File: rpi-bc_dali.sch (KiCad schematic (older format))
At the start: 5 parts, among them J1 Raspberry_Pi_2_3, J2 Conn_01x04, J3 Conn_01x04, J4 Conn_01x04, J5 Conn_01x04

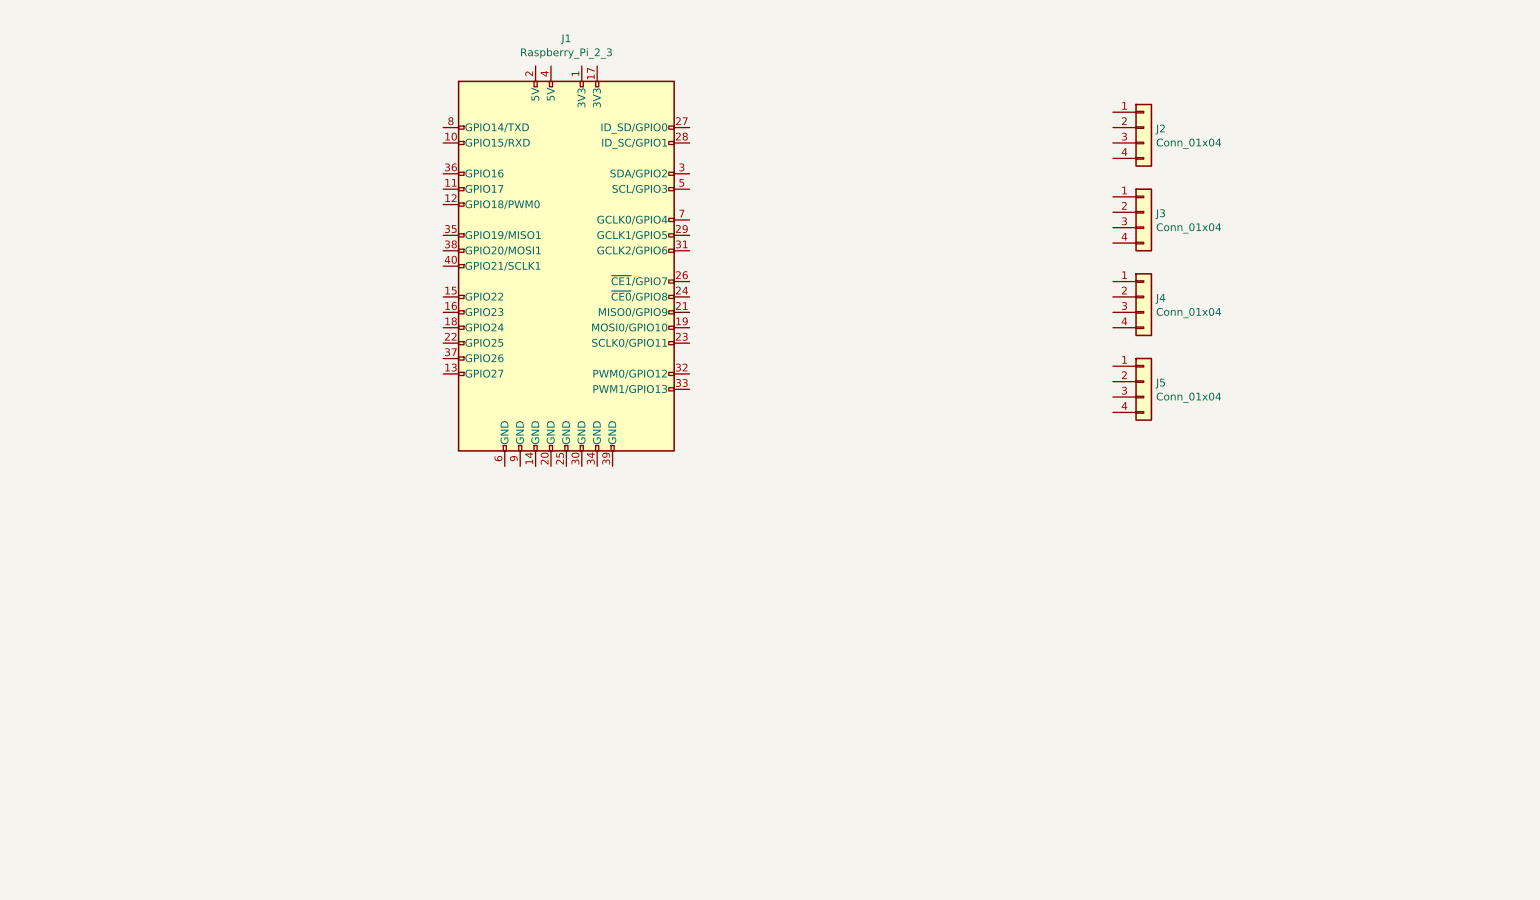
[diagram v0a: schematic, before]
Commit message: master : schematic update
 - first pass schematic.
 - annotated.
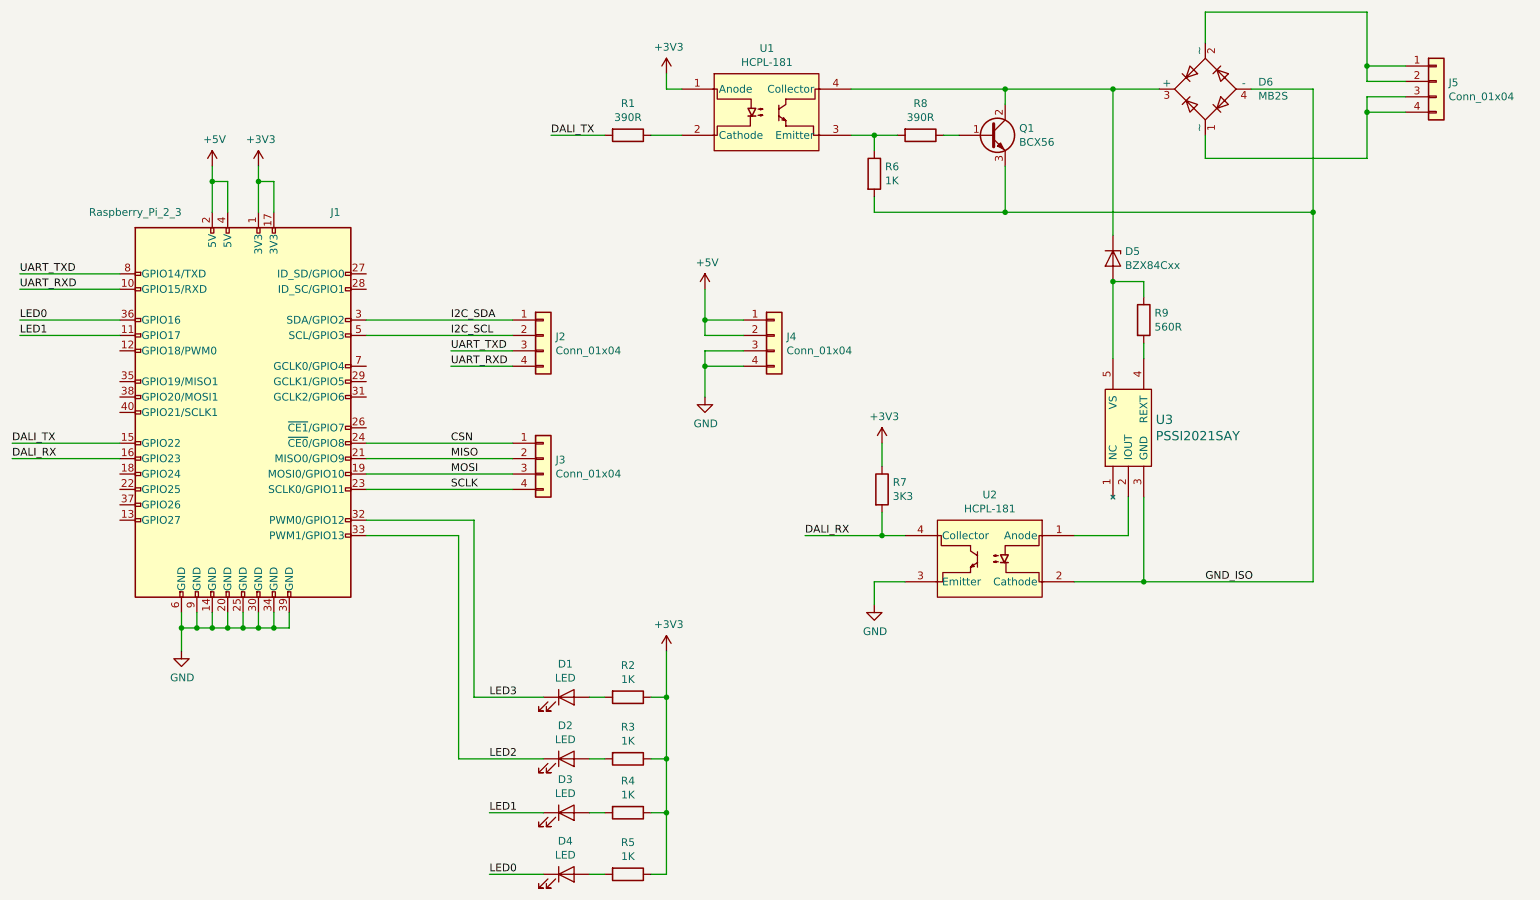
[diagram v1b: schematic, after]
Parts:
- added D1, D2, D3, D4: LED, symbol Device:LED
- added D5: BZX84Cxx, Diode_SMD:D_SOT-23_ANK, symbol Diode:BZX84Cxx
- added D6: MB2S, Package_TO_SOT_SMD:TO-269AA, symbol Diode_Bridge:MB2S
- added Q1: BCX56, Package_TO_SOT_SMD:SOT-89-3, symbol Transistor_BJT:BCX56
- added R1, R8: 390R, symbol Device:R
- added R2, R3, R4, R5, R6: 1K, symbol Device:R
- added R7: 3K3, symbol Device:R
- added R9: 560R, symbol Device:R
- added U1, U2: HCPL-181, symbol Isolator:HCPL-181
- added U3: PSSI2021SAY, symbol Reference_Current:PSSI2021SAY
- renumbered J4 to J2, J5 to J4, J2 to J5
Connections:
- net at J5.1 (Pin_1): now also J5.2 (Pin_2), D6.2 (~~)
- net at J5.3 (Pin_3): now also J5.4 (Pin_4), D6.1 (~~)
- net CSN: now reaches J3.1 (Pin_1)
- net CSN: now also J1.24 (~CE0~/GPIO8)
- net MISO: now reaches J3.2 (Pin_2)
- net MISO: now also J1.21 (MISO0/GPIO9)
- net MOSI: now reaches J3.3 (Pin_3)
- net MOSI: now also J1.19 (MOSI0/GPIO10)
- net SCLK: now reaches J3.4 (Pin_4)
- net SCLK: now also J1.23 (SCLK0/GPIO11)
- net I2C_SDA: now reaches J2.1 (Pin_1)
- net I2C_SDA: now also J1.3 (SDA/GPIO2)
- net I2C_SCL: now reaches J2.2 (Pin_2)
- net I2C_SCL: now also J1.5 (SCL/GPIO3)
- net UART_TXD: now reaches J2.3 (Pin_3)
- net UART_TXD: now also J1.8 (GPIO14/TXD)
- net UART_RXD: now reaches J2.4 (Pin_4)
- net UART_RXD: now also J1.10 (GPIO15/RXD)
- net +5V: now reaches J4.1 (Pin_1)
- net +5V: now also J1.2 (5V), J1.4 (5V), J4.2 (Pin_2)
- net GND: now reaches J4.3 (Pin_3)
- net GND: now also J1.14 (GND), J1.20 (GND), J1.25 (GND), J1.30 (GND), J1.34 (GND), J1.39 (GND), J1.6 (GND), J1.9 (GND), J4.4 (Pin_4), U2.3 (Emitter)
- net +3V3: now reaches J1.1 (3V3)
- net +3V3: now also J1.17 (3V3), R2.1, R3.1, R4.1, R5.1, R7.1, U1.1 (Anode)
- net LED1: now reaches J1.11 (GPIO17)
- net LED1: now also D3.1 (K)
- net DALI_TX: now reaches J1.15 (GPIO22)
- net DALI_TX: now also R1.2
- net DALI_RX: now reaches J1.16 (GPIO23)
- net DALI_RX: now also R7.2, U2.4 (Collector)
- net LED3: now reaches J1.32 (PWM0/GPIO12)
- net LED3: now also D1.1 (K)
- net LED2: now reaches J1.33 (PWM1/GPIO13)
- net LED2: now also D2.1 (K)
- net LED0: now reaches J1.36 (GPIO16)
- net LED0: now also D4.1 (K)
- new net: R1.1, U1.2 (Cathode)
- new net: R6.1, R8.2, U1.3 (Emitter)
- new net: D5.1 (K), D6.3 (+), Q1.2 (C), U1.4 (Collector)
- new net: U2.1 (Anode), U3.2 (IOUT)
- new net: R9.2, U3.4 (REXT)
- new net: D5.2 (A), R9.1, U3.5 (VS)
- new net: Q1.1 (B), R8.1
- new net: D1.2 (A), R2.2
- new net: D2.2 (A), R3.2
- new net: D3.2 (A), R4.2
- new net: D4.2 (A), R5.2
- new net GND_ISO: D6.4 (-), Q1.3 (E), R6.2, U2.2 (Cathode), U3.3 (GND)
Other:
- moved on the sheet: J1, J2, J3, J4, J5
